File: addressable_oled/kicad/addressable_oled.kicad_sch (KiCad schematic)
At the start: 21 parts, among them J1 Conn_01x05_Pin, J2 Conn_01x03_Socket, U1 SLG46826G, U2 OLED-128O064D

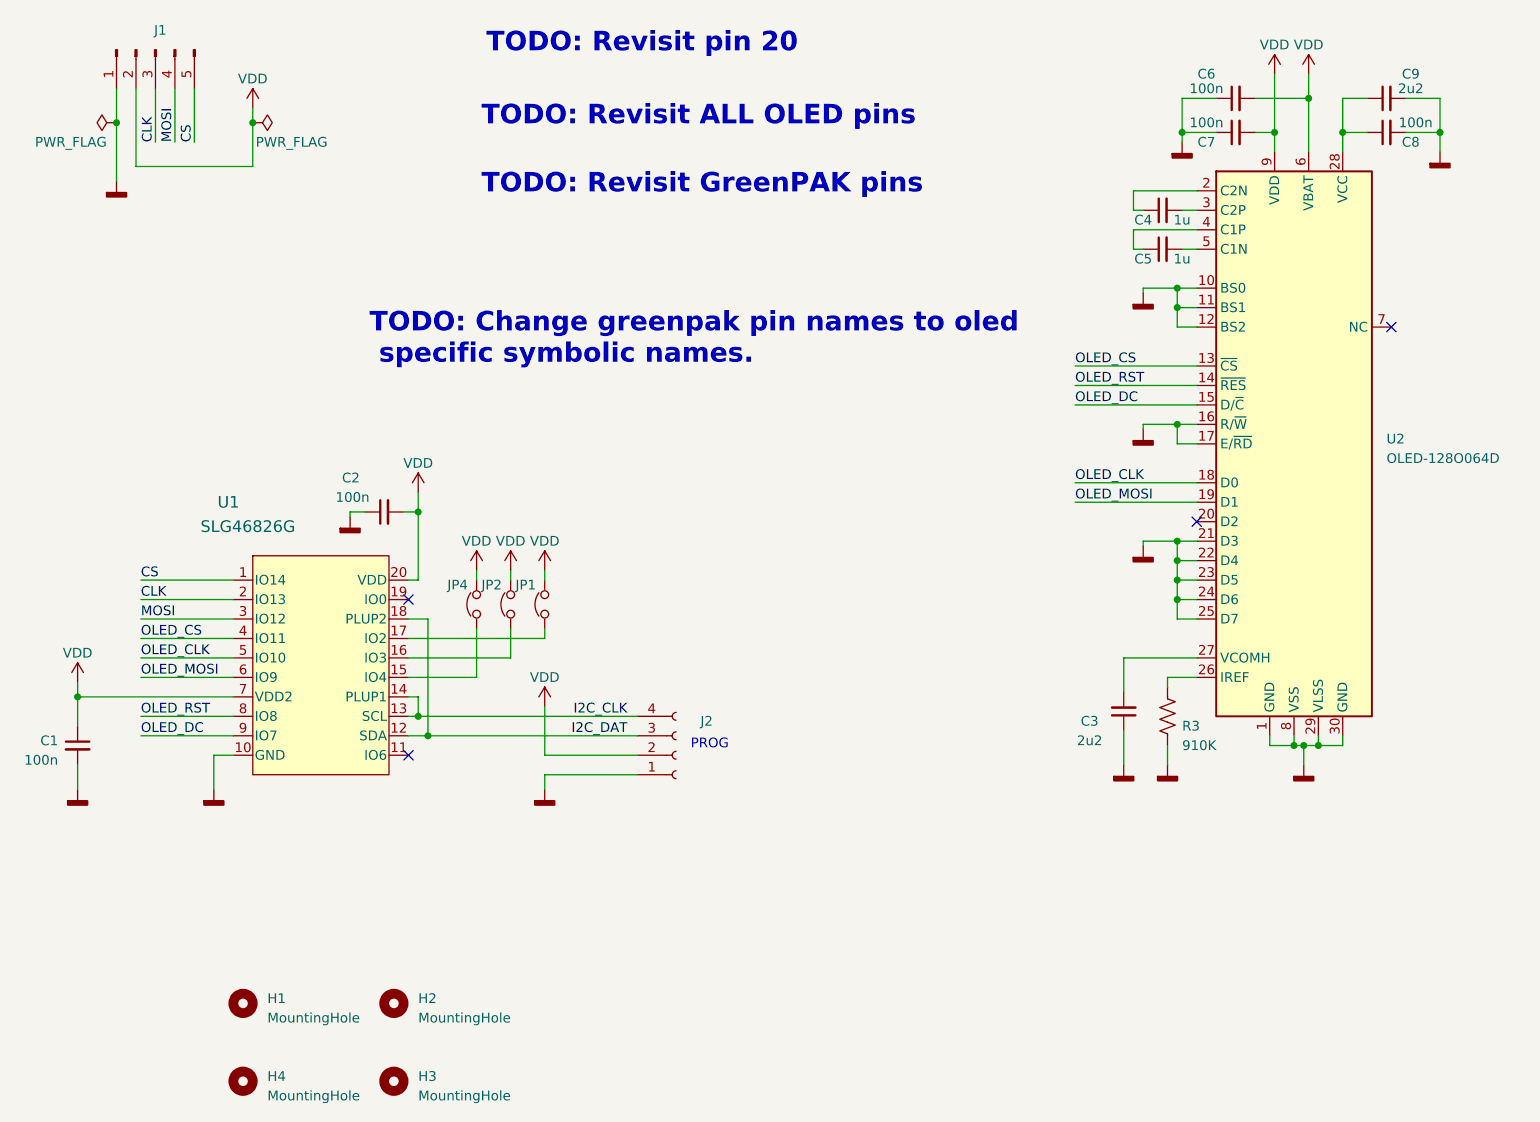
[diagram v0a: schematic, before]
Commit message: Final cleanup.
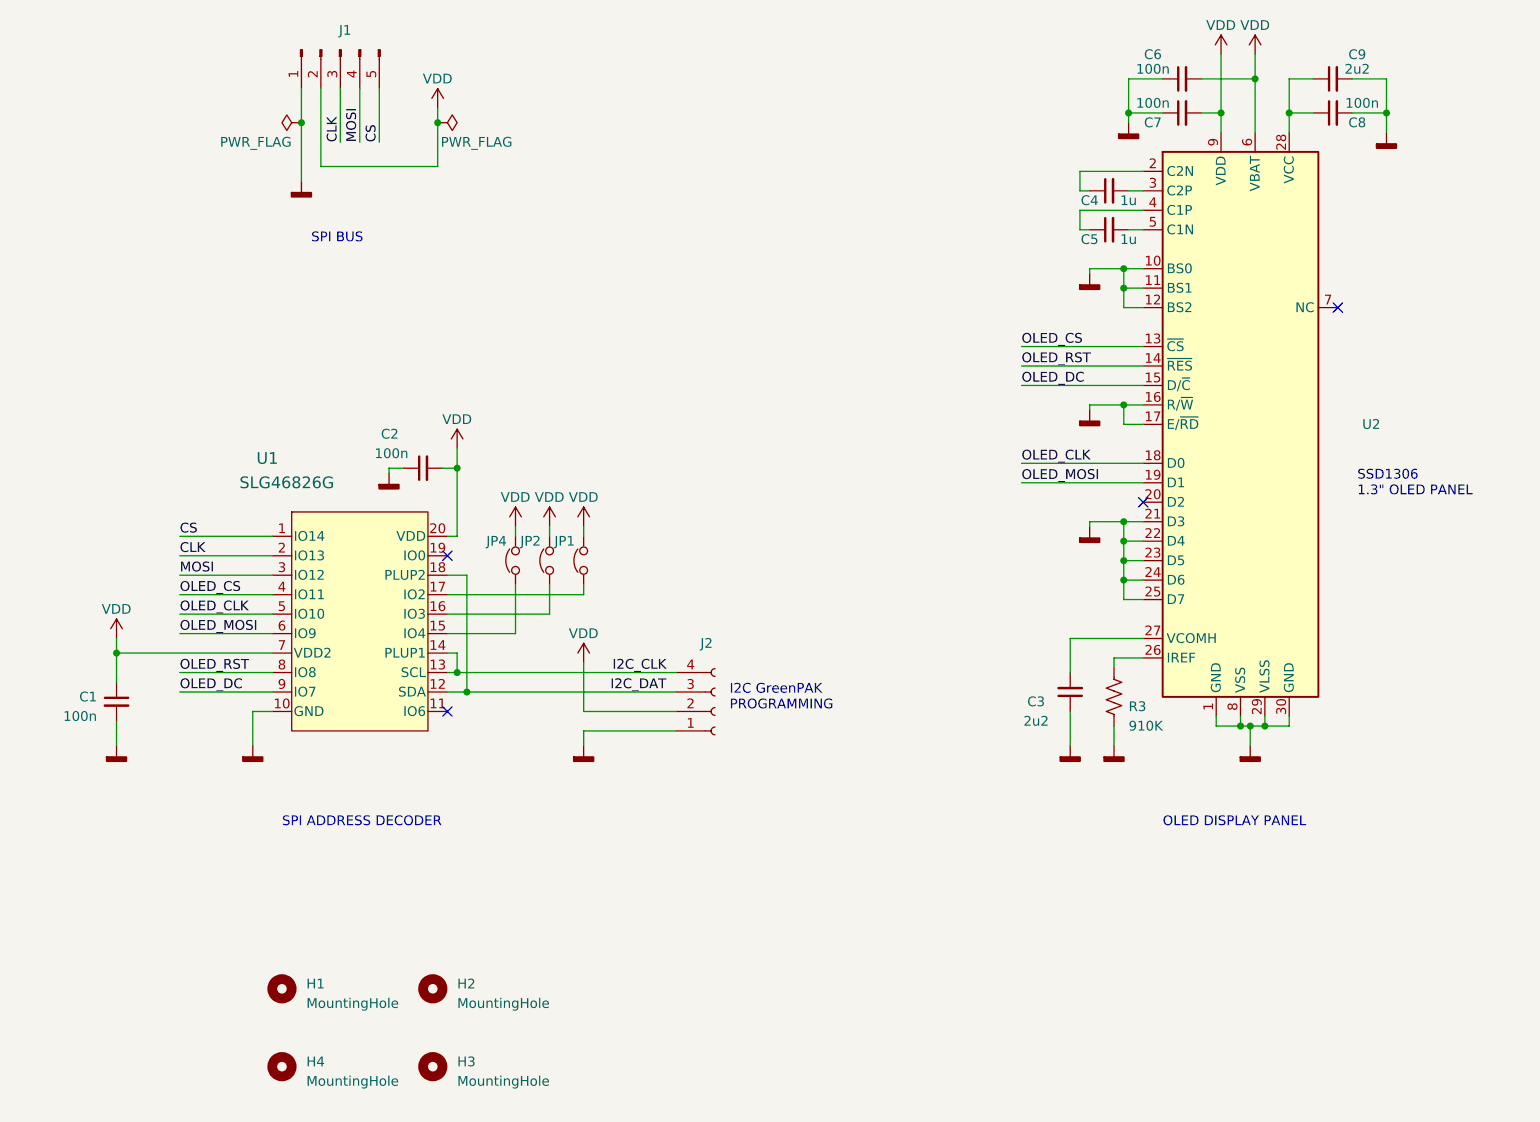
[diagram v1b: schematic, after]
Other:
- note added: "I2C GreenPAK PROGRAMMING"
- note added: "OLED DISPLAY PANEL"
- note added: "SPI ADDRESS DECODER"
- note added: "SPI BUS"
- note added: "SSD1306 1.3" OLED PANEL"
- note removed: "PROG"
- note removed: "TODO: Change greenpak pin names to oled specific symbolic names."
- note removed: "TODO: Revisit ALL OLED pins"
- note removed: "TODO: Revisit GreenPAK pins"
- note removed: "TODO: Revisit pin 20"
- title: (none) -> ADDRESSABLE SPI OLED
- moved on the sheet: C1, C2, C3, C4, C5, C6, C7, C8, C9, H1, H2, H3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
